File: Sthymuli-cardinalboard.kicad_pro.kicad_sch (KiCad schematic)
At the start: 38 parts, among them J8 Conn_02x08_Counter_Clockwise, Q10 NX7002AK, Q11 NX7002AK, Q12 NX7002AK, Q13 NX7002AK, SW10 SW_Push, SW7 SW_Push, SW8 SW_Push, SW9 SW_Push, U13 LSM6DS3, U17 ITR9909, U18 ITR9909, U19 ITR9909, U20 ITR9909

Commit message: routing small board
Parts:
- removed Q12, Q13: NX7002AK, Package_TO_SOT_SMD:SOT-23, symbol Transistor_FET_Other:Q_NMOS_Depletion_GSD
- removed R54, R55: 3K3, Capacitor_SMD:C_0201_0603Metric, symbol Device:R
- removed R64, R65: 27R, Capacitor_SMD:C_0201_0603Metric, symbol Device:R
- removed SW10, SW9: SW_Push, sthymuli:XKB5858, symbol Switch:SW_Push
- removed U19, U20: ITR9909, sthymuli:ITR_9909_Vertical, symbol kitprisme:ITR9909
- J1: renamed from J8; footprint (none) -> Connector_PinSocket_2.54mm:PinSocket_2x08_P2.54mm_Vertical_SMD
- U2: renamed from U18; footprint sthymuli:ITR_9909_Horizontal -> sthymuli:ITR_9909_Vertical
- renumbered C20 to C1, C21 to C2, C22 to C3, C23 to C4, C24 to C5, C25 to C6, C77 to C7, D20 to D1, D26 to D2, D21 to D3, D22 to D4, D23 to D5, D24 to D6, D25 to D7, Q10 to Q1, Q11 to Q2, R52 to R1, R53 to R2, R62 to R3, R63 to R4, SW7 to SW1, SW8 to SW2, U17 to U1, U13 to U3
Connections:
- net ACC_B_INT1 is gone; now on net +3V3: J1.2 (Pin_2)
- net btn_EAST_DOWN is gone; now on net btn_DOWN: J1.4 (Pin_4)
- net btn_EAST_UP is gone; now on net IR_TRA_VERT: J1.13 (Pin_13)
- net +3V3: no longer J1.1 (Pin_1)
- net +5V: now also J1.1 (Pin_1); no longer J1.16 (Pin_16)
- net BAT+: now also J1.6 (Pin_6); no longer J1.7 (Pin_7)
- net BAT-: now also J1.7 (Pin_7); no longer J1.10 (Pin_10)
- net DIN: now also J1.8 (Pin_8); no longer J1.3 (Pin_3)
- net DOUT: now also J1.9 (Pin_9); no longer J1.14 (Pin_14)
- net GND: now also J1.3 (Pin_3); no longer J1.15 (Pin_15)
- net SCL: now also J1.15 (Pin_15); no longer J1.9 (Pin_9)
- net SDA: now also J1.14 (Pin_14); no longer J1.8 (Pin_8)
- net btn_UP: now also J1.5 (Pin_5)
- net ACC_INT: now reaches U3.4 (INT1)
- net ACC_INT: now also J1.16 (Pin_16)
- net IR_REC_2 renamed IR_REC_HORI
- net IR_REC_HORI: now also J1.10 (Pin_10); no longer J1.5 (Pin_5)
- net IR_REC_3 renamed IR_REC_VERT
- net IR_REC_VERT: now also J1.12 (Pin_12); no longer J1.6 (Pin_6)
- net IR_TRA_2 renamed IR_TRA_HORI
- net IR_TRA_HORI: now also J1.11 (Pin_11); no longer J1.12 (Pin_12)
- net IR_TRA_3 renamed IR_TRA_VERT
- net IR_TRA_VERT: no longer J1.11 (Pin_11)
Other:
- note removed: "Buttons/switch"
- note removed: "we use MCP23017 internal pull-ups"
- moved on the sheet: BT1, C1, C2, C3, C4, C5, C6, C7, D1, D2, D3, D4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

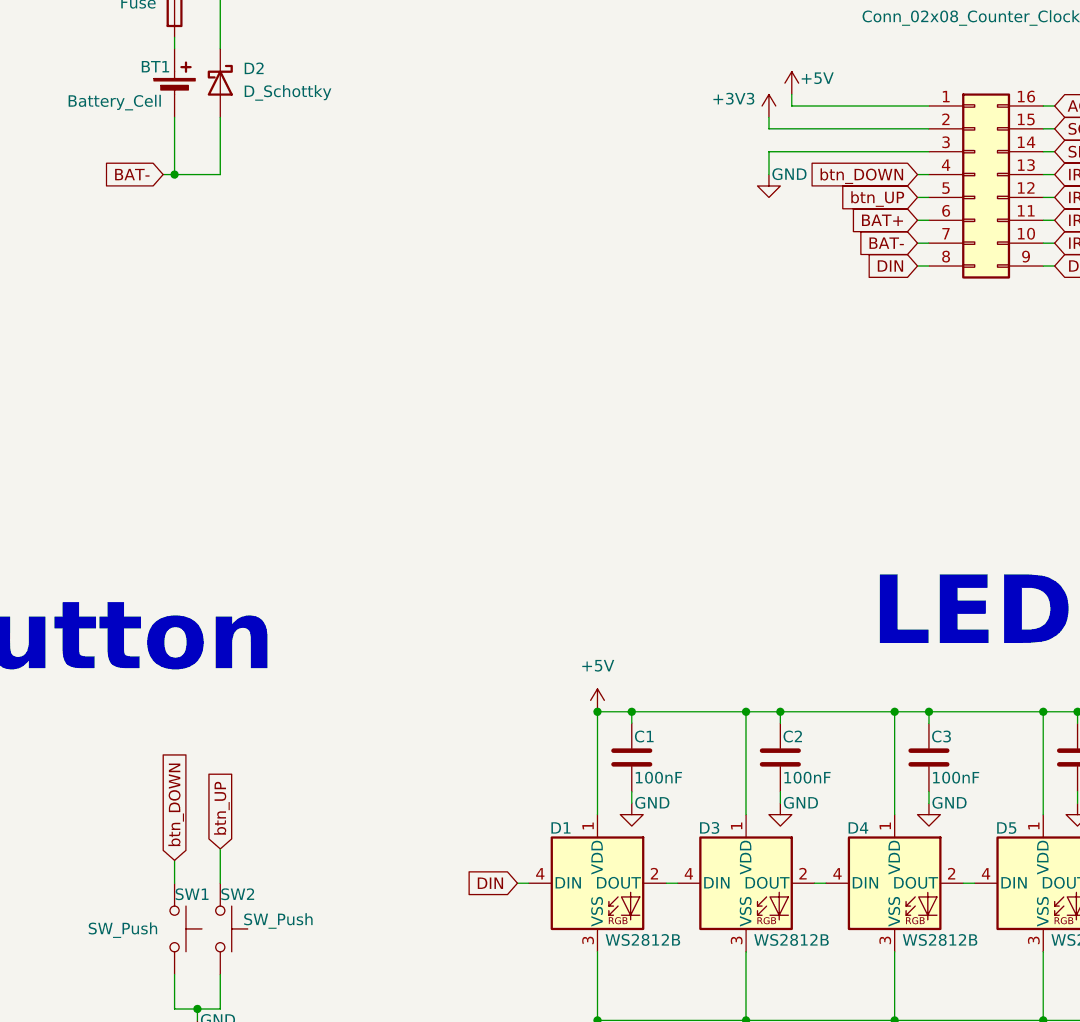
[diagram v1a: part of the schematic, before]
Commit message: tried autoroute...
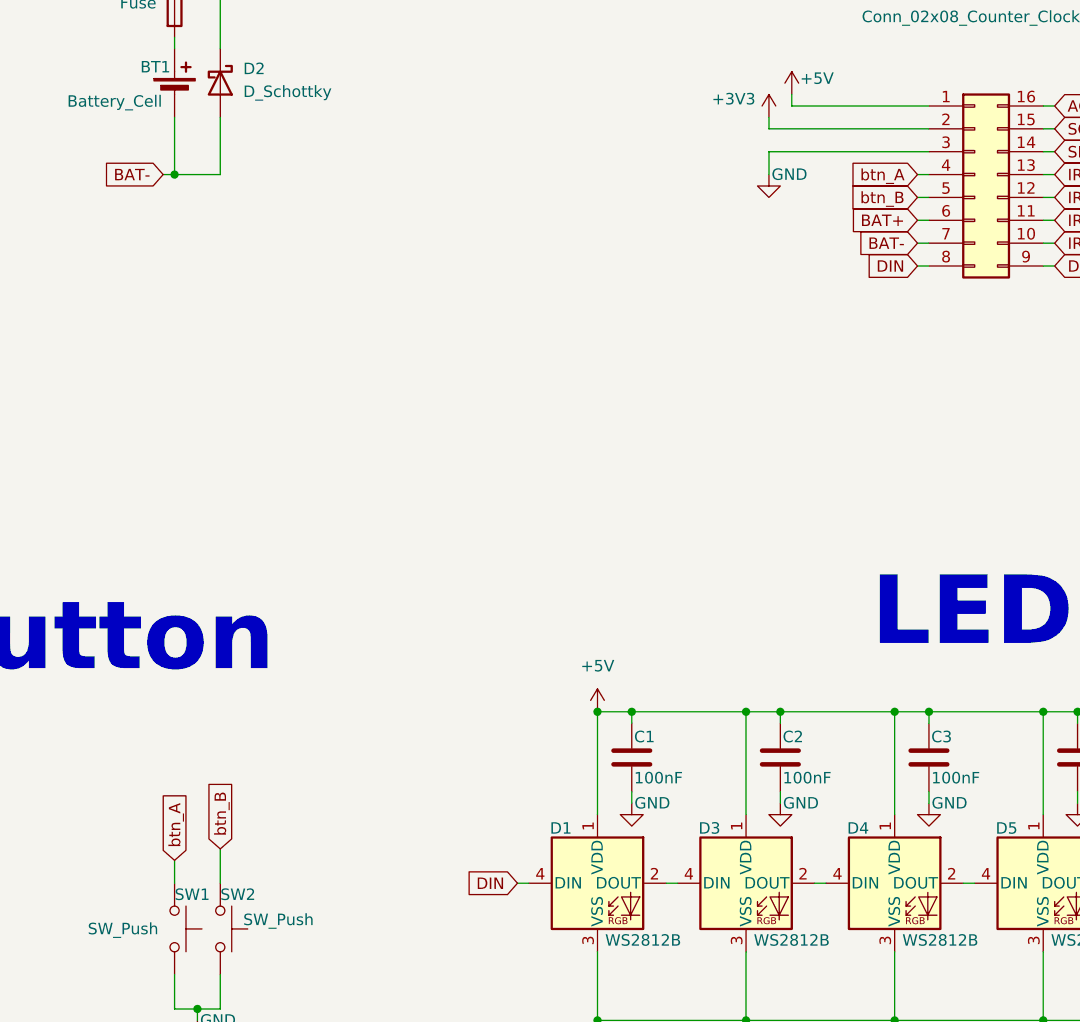
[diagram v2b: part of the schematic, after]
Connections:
- net btn_DOWN renamed btn_A
- net btn_UP renamed btn_B
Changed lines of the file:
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@@
 		)
 	)
-	(global_label "btn_DOWN"
+	(global_label "btn_A"
 		(shape input)
 		(at 48.26 142.24 90)
@@
 		)
 		(property "Intersheetrefs" "${INTERSHEET_REFS}"
-			(at 48.26 129.8811 90)
+			(at 48.26 134.1749 90)
 			(hide yes)
 			(show_name no)
@@
 		)
 	)
-	(global_label "btn_UP"
+	(global_label "btn_B"
 		(shape input)
 		(at 53.34 140.97 90)
@@
 		)
 		(property "Intersheetrefs" "${INTERSHEET_REFS}"
-			(at 53.34 131.393 90)
+			(at 53.34 132.7235 90)
 			(hide yes)
 			(show_name no)
@@
 		)
 	)
-	(global_label "btn_DOWN"
+	(global_label "btn_A"
 		(shape input)
 		(at 130.81 66.04 180)
@@
 		)
 		(property "Intersheetrefs" "${INTERSHEET_REFS}"
-			(at 118.4511 66.04 0)
+			(at 122.7449 66.04 0)
 			(hide yes)
 			(show_name no)
@@
 		)
 	)
-	(global_label "btn_UP"
+	(global_label "btn_B"
 		(shape input)
 		(at 130.81 68.58 180)
@@
 		)
 		(property "Intersheetrefs" "${INTERSHEET_REFS}"
-			(at 121.233 68.58 0)
-			(hide yes)
-			(show_name no)
+			(at 122.5635 68.58 0)
+			(hide yes)
+			(show_name no)
